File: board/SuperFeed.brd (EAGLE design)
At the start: 97.8 x 59.7 mm, 16 parts

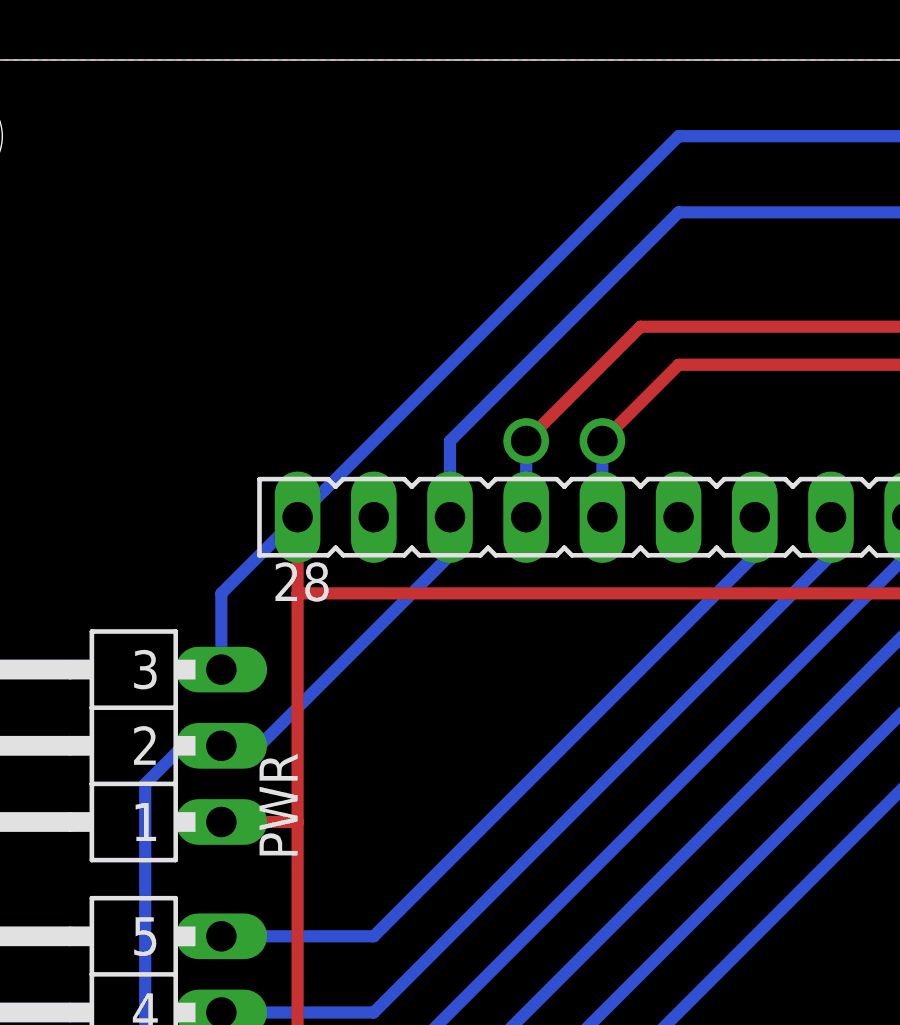
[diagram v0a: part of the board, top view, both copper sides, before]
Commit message: Minor improvement in the board
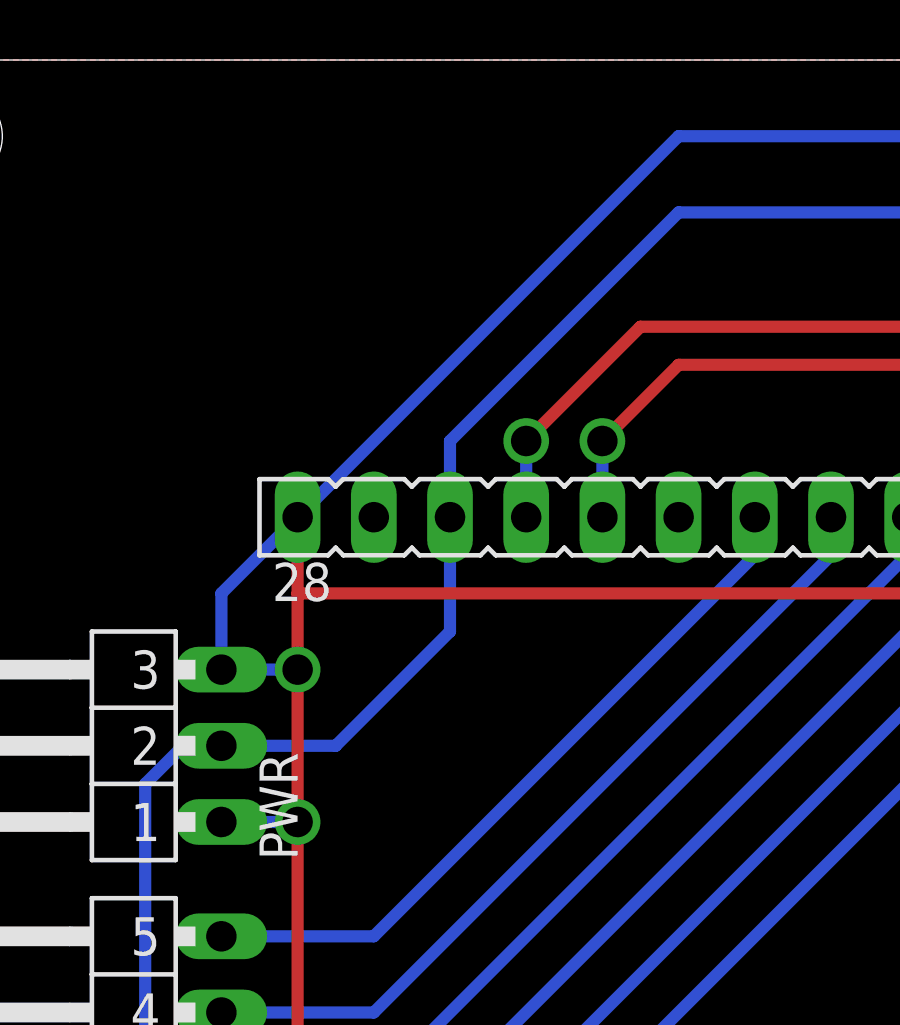
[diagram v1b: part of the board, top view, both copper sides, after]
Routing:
- net +5V: track 242.0 -> 244.7 mm
- net GND: track 277.1 -> 279.6 mm, vias 1 -> 3
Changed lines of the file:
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@@
 <layer number="42" name="bRestrict" color="1" fill="10" visible="yes" active="yes"/>
 <layer number="43" name="vRestrict" color="2" fill="10" visible="yes" active="yes"/>
-<layer number="44" name="Drills" color="7" fill="1" visible="no" active="yes"/>
+<layer number="44" name="Drills" color="7" fill="1" visible="yes" active="yes"/>
 <layer number="45" name="Holes" color="7" fill="1" visible="no" active="yes"/>
 <layer number="46" name="Milling" color="3" fill="1" visible="yes" active="yes"/>
@@
 <wire x1="13.97" y1="13.97" x2="13.97" y2="17.78" width="0.4064" layer="16"/>
 <wire x1="13.97" y1="17.78" x2="11.43" y2="20.32" width="0.4064" layer="16"/>
-<wire x1="11.43" y1="39.37" x2="11.43" y2="41.91" width="0.4064" layer="16"/>
-<wire x1="11.43" y1="41.91" x2="13.97" y2="44.45" width="0.4064" layer="16"/>
 <wire x1="49.53" y1="57.15" x2="26.67" y2="57.15" width="0.4064" layer="16"/>
 <wire x1="82.55" y1="13.97" x2="82.55" y2="10.16" width="0.4064" layer="16"/>
@@
 <wire x1="82.55" y1="13.97" x2="82.55" y2="41.91" width="0.4064" layer="1"/>
 <wire x1="13.97" y1="13.97" x2="13.97" y2="34.29" width="0.4064" layer="1"/>
-<wire x1="13.97" y1="34.29" x2="13.97" y2="41.91" width="0.4064" layer="1"/>
+<wire x1="13.97" y1="39.37" x2="13.97" y2="41.91" width="0.4064" layer="1"/>
 <wire x1="13.97" y1="41.91" x2="71.12" y2="41.91" width="0.4064" layer="1"/>
-<wire x1="26.67" y1="57.15" x2="13.97" y2="44.45" width="0.4064" layer="16"/>
 <contactref element="R1" pad="3"/>
 <wire x1="82.55" y1="44.45" x2="86.36" y2="44.45" width="0.4064" layer="16"/>
@@
 <wire x1="71.12" y1="57.15" x2="71.12" y2="41.91" width="0.4064" layer="16"/>
 <via x="71.12" y="41.91" extent="1-16" drill="1.016"/>
+<wire x1="82.55" y1="44.45" x2="82.55" y2="41.91" width="0.4064" layer="1"/>
+<wire x1="82.55" y1="41.91" x2="71.12" y2="41.91" width="0.4064" layer="1"/>
+<wire x1="13.97" y1="44.45" x2="13.97" y2="41.91" width="0.4064" layer="1"/>
+<contactref element="PWR" pad="1"/>
+<contactref element="EXTBTN" pad="5"/>
+<wire x1="34.29" y1="3.81" x2="36.83" y2="6.35" width="0.4064" layer="16"/>
+<wire x1="17.78" y1="6.35" x2="17.78" y2="5.08" width="0.4064" layer="16"/>
+<wire x1="17.78" y1="5.08" x2="19.05" y2="3.81" width="0.4064" layer="16"/>
+<wire x1="19.05" y1="3.81" x2="34.29" y2="3.81" width="0.4064" layer="16"/>
+<wire x1="11.43" y1="34.29" x2="13.97" y2="34.29" width="0.4064" layer="16"/>
+<via x="13.97" y="34.29" extent="1-16" drill="1.016"/>
+<wire x1="11.43" y1="39.37" x2="13.97" y2="39.37" width="0.4064" layer="16"/>
+<via x="13.97" y="39.37" extent="1-16" drill="1.016"/>
+<wire x1="13.97" y1="39.37" x2="13.97" y2="34.29" width="0.4064" layer="1"/>
+<wire x1="13.97" y1="44.45" x2="11.43" y2="41.91" width="0.4064" layer="16"/>
+<wire x1="11.43" y1="39.37" x2="11.43" y2="41.91" width="0.4064" layer="16"/>
+<wire x1="13.97" y1="44.45" x2="26.67" y2="57.15" width="0.4064" layer="16"/>
 <polygon width="0.4064" layer="1" isolate="0.4064" orphans="yes" rank="6">
 <vertex x="97.79" y="59.69"/>
@@
 <vertex x="0" y="59.69"/>
 </polygon>
-<wire x1="82.55" y1="44.45" x2="82.55" y2="41.91" width="0.4064" layer="1"/>
-<wire x1="82.55" y1="41.91" x2="71.12" y2="41.91" width="0.4064" layer="1"/>
-<wire x1="13.97" y1="44.45" x2="13.97" y2="41.91" width="0.4064" layer="1"/>
-<contactref element="PWR" pad="1"/>
-<wire x1="11.43" y1="34.29" x2="13.97" y2="34.29" width="0.4064" layer="1"/>
-<contactref element="EXTBTN" pad="5"/>
-<wire x1="34.29" y1="3.81" x2="36.83" y2="6.35" width="0.4064" layer="16"/>
-<wire x1="17.78" y1="6.35" x2="17.78" y2="5.08" width="0.4064" layer="16"/>
-<wire x1="17.78" y1="5.08" x2="19.05" y2="3.81" width="0.4064" layer="16"/>
-<wire x1="19.05" y1="3.81" x2="34.29" y2="3.81" width="0.4064" layer="16"/>
 </signal>
 <signal name="+5V">
@@
 <wire x1="13.97" y1="2.54" x2="73.66" y2="2.54" width="0.4064" layer="16"/>
 <wire x1="73.66" y1="2.54" x2="77.47" y2="2.54" width="0.4064" layer="16"/>
-<wire x1="11.43" y1="36.83" x2="12.7" y2="36.83" width="0.4064" layer="16"/>
-<wire x1="12.7" y1="36.83" x2="19.05" y2="43.18" width="0.4064" layer="16"/>
 <wire x1="19.05" y1="43.18" x2="19.05" y2="44.45" width="0.4064" layer="16"/>
 <wire x1="52.07" y1="57.15" x2="52.07" y2="55.88" width="0.4064" layer="16"/>
@@
 <via x="85.09" y="52.07" extent="1-16" drill="1.016"/>
 <wire x1="85.09" y1="52.07" x2="52.07" y2="52.07" width="0.4064" layer="1"/>
+<wire x1="11.43" y1="36.83" x2="15.24" y2="36.83" width="0.4064" layer="16"/>
+<wire x1="15.24" y1="36.83" x2="19.05" y2="40.64" width="0.4064" layer="16"/>
+<wire x1="19.05" y1="40.64" x2="19.05" y2="44.45" width="0.4064" layer="16"/>
 </signal>
 <signal name="NC">
